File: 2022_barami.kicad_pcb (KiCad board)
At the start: 4 copper layers, 95.2 x 139.7 mm, 10 parts, among them J1 GM7123 Module, J2 External IO, U1 NUCLEO144-H743ZI, U2 23LC1024-E/P

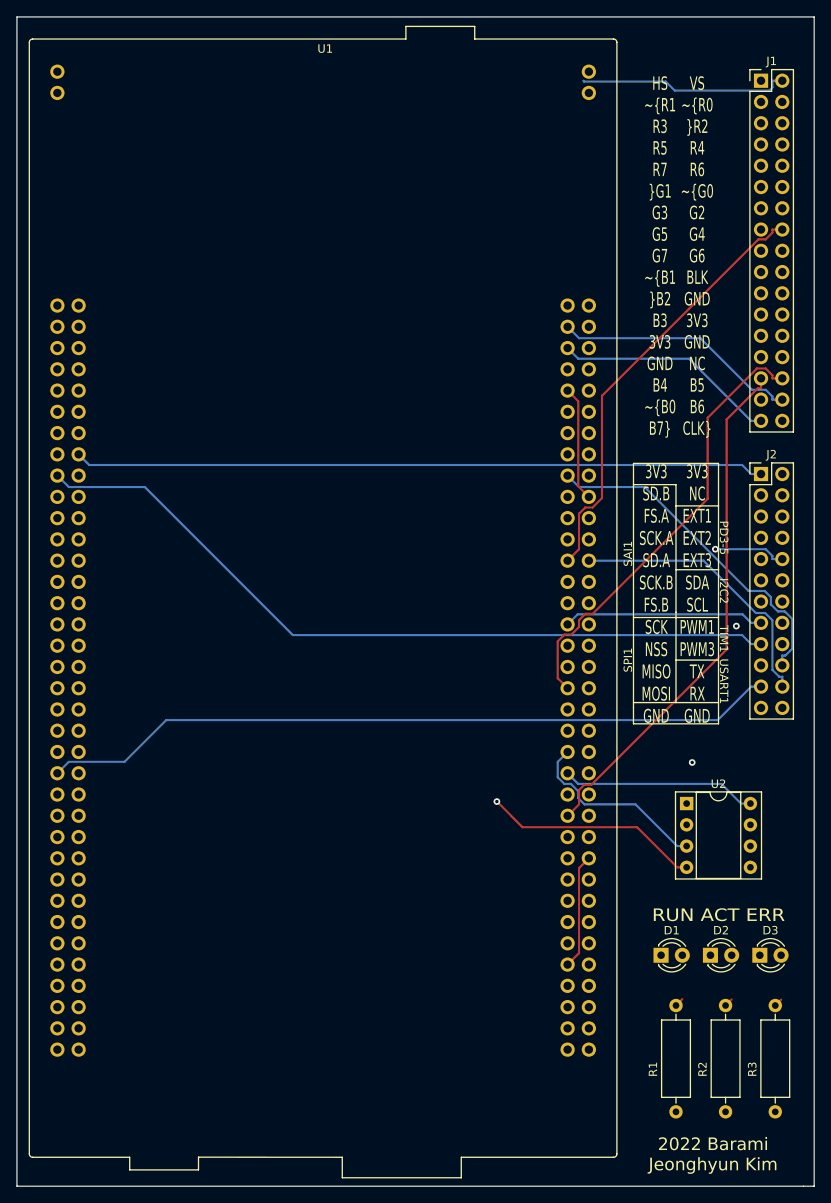
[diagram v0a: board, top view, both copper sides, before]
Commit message: Update schemetic with KiCAD files
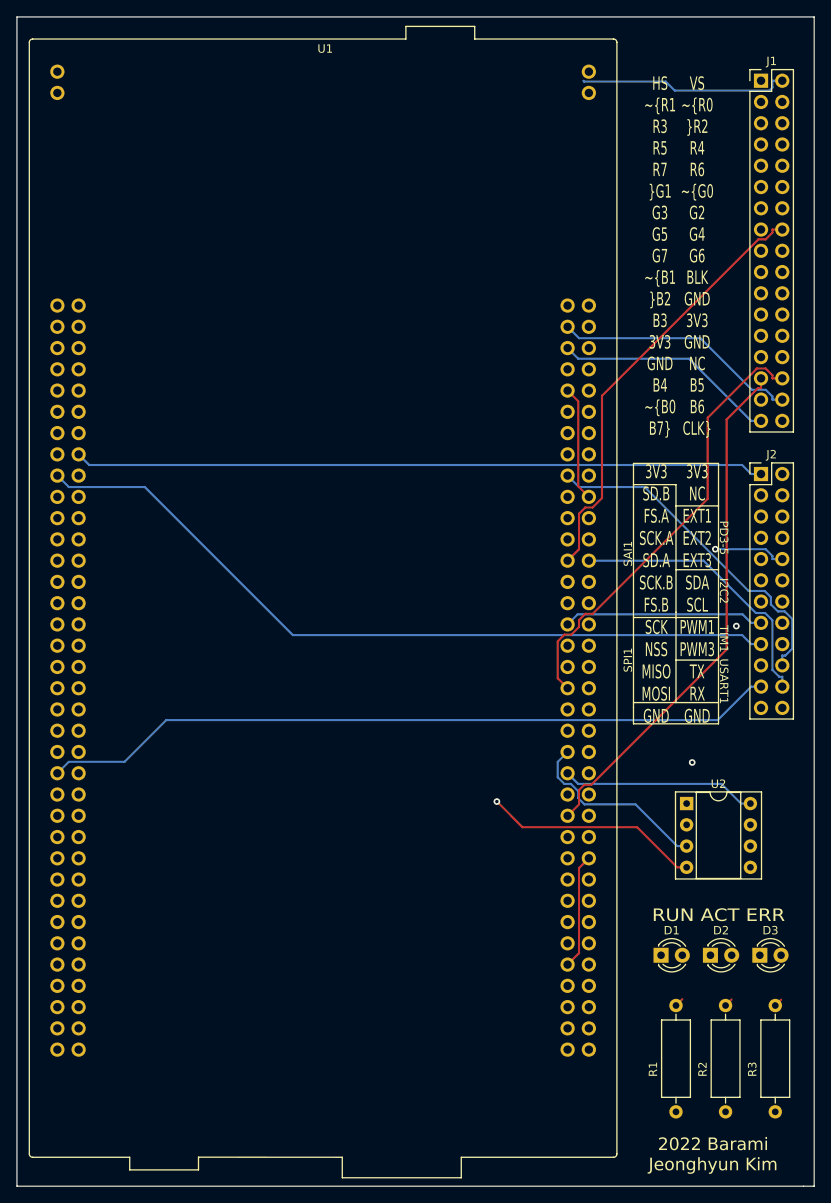
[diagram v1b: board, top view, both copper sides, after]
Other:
- net class Default removed
- board text added: "HS ~{R1 R3 R5 R7 }G1 G3 G5 G7 ~{B1 }B2 B3 3V3 GND B4 ~{B0 B7}"
- board text added: "VS ~{R0 }R2 R4 R6 ~{G0 G2 G4 G6 BLK GND 3V3 GND NC B5 B6 CLK}"
- board text removed: "HS ~R1 R3 R5 R7 ~G1 G3 G5 G7 ~B1 ~B2 B3 3V3 GND B4 ~B0 B7"
- board text removed: "VS ~R0 ~R2 R4 R6 ~G0 G2 G4 G6 BLK GND 3V3 GND NC B5 B6 CLK"
